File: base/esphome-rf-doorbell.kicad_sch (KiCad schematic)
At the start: 93 parts, among them J1 B4B-XH, J2 CONUFL001-SMD-T, J3 Conn_01x01, J4 Conn_01x01, SW1 Boot, U1 BQ25628E, U2 RFM69W, U3 TPS7A2033, U4 MAX17261xxTD, U5 TPS629206DRLR, U6 G3VM-31DR, U7 ESP32-S2-MINI-2, U8 G3VM-63ER, U9 TLP2391

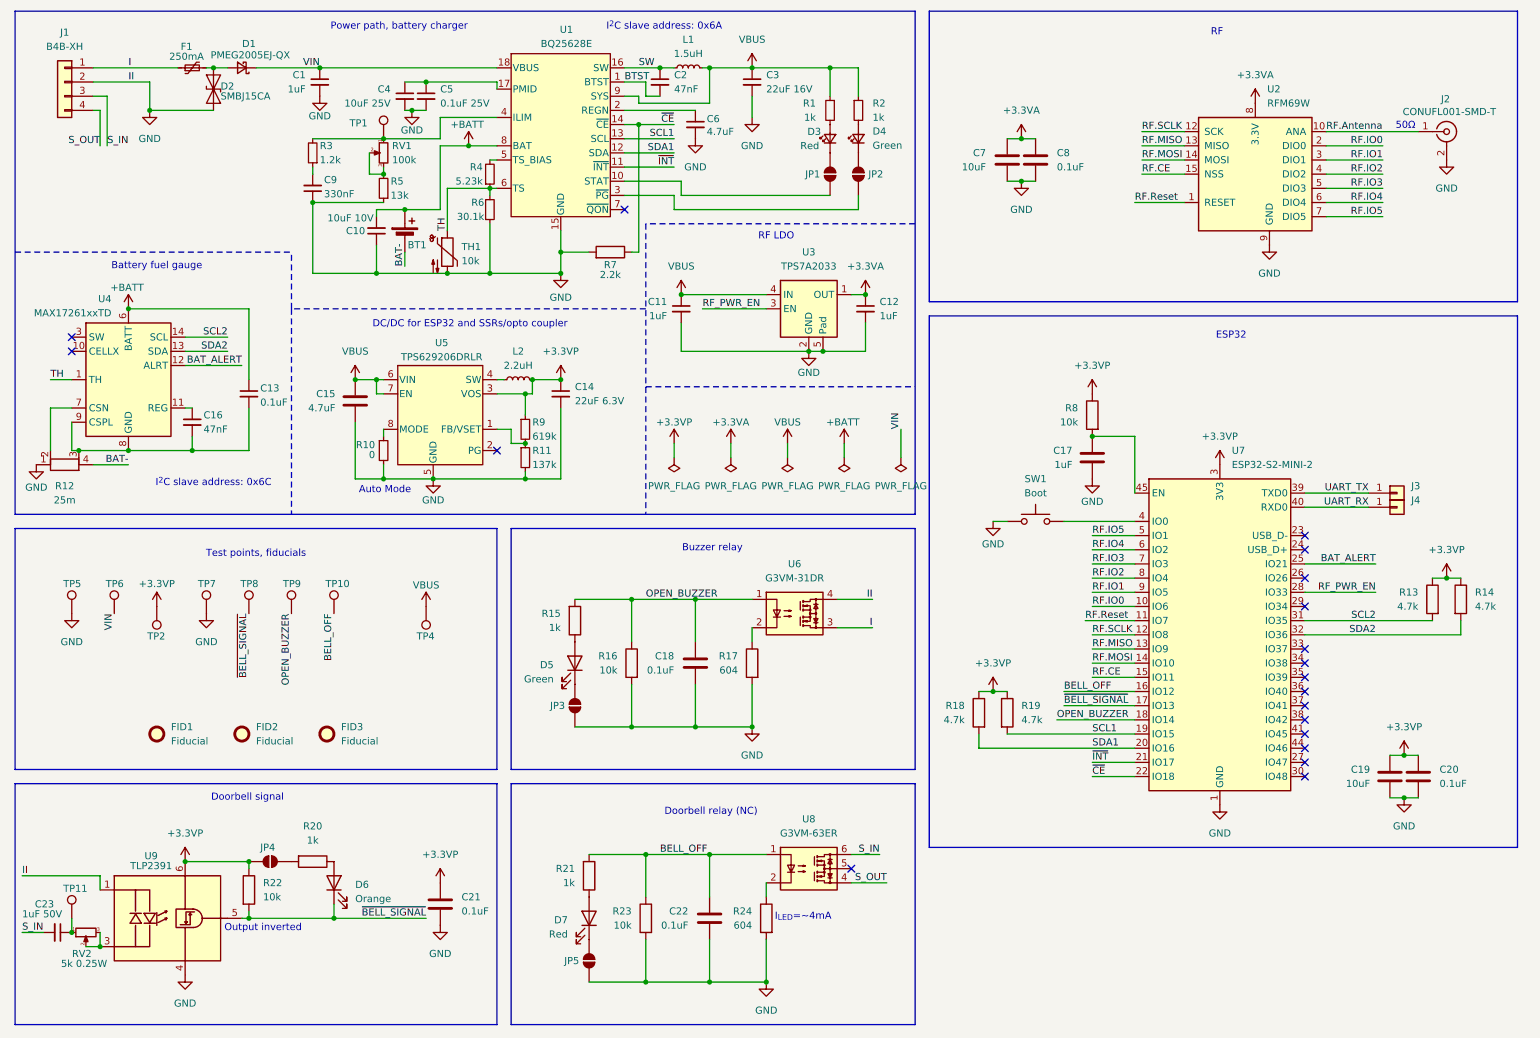
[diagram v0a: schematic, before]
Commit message: Base board Rev3
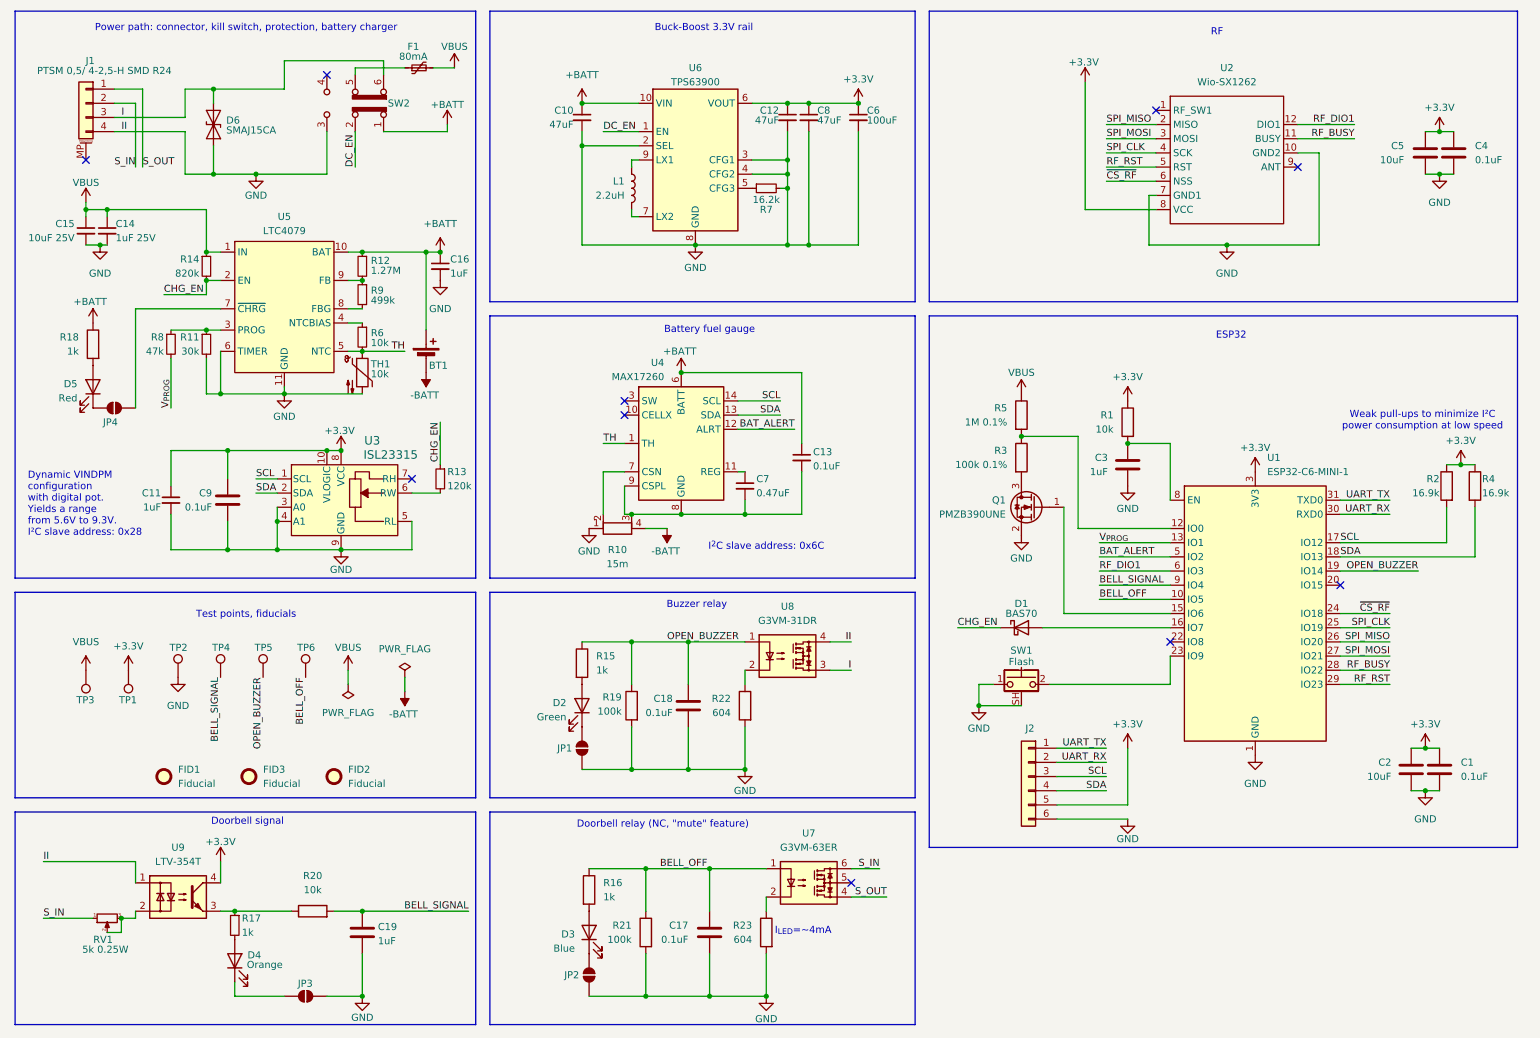
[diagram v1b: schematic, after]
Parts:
- removed C1: 1uF, Capacitor_SMD:C_0402_1005Metric, symbol Device:C_Small
- removed C15: 4.7uF, Capacitor_SMD:C_0603_1608Metric, symbol Device:C
- removed C2: 47nF, Capacitor_SMD:C_0402_1005Metric, symbol Device:C_Small
- removed C21: 0.1uF, Capacitor_SMD:C_0402_1005Metric, symbol Device:C
- removed C23: 1uF 50V, Capacitor_SMD:C_0805_2012Metric, symbol Device:C_Small
- removed C3: 22uF 16V, Capacitor_SMD:C_0805_2012Metric, symbol Device:C_Small
- removed C4: 10uF 25V, Capacitor_SMD:C_0603_1608Metric, symbol Device:C_Small
- removed C5: 0.1uF 25V, Capacitor_SMD:C_0402_1005Metric, symbol Device:C_Small
- removed C9: 330nF, Capacitor_SMD:C_0402_1005Metric, symbol Device:C_Small
- removed D1: PMEG2005EJ-QX, Diode_SMD:D_SOD-323F, symbol Device:D_Schottky_Small
- removed D3: Red, LED_SMD:LED_0603_1608Metric, symbol Device:LED_Small
- removed D4: Green, LED_SMD:LED_0603_1608Metric, symbol Device:LED_Small
- removed J1: B4B-XH, Connector_JST:JST_XH_B4B-XH-A_1x04_P2.50mm_Vertical, symbol Connector_Generic:Conn_01x04
- removed J2: CONUFL001-SMD-T, Connector_Coaxial:U.FL_Hirose_U.FL-R-SMT-1_Vertical, symbol Connector:Conn_Coaxial
- removed J3, J4: Conn_01x01, TestPoint:TestPoint_Keystone_5000-5004_Miniature, symbol Connector_Generic:Conn_01x01
- removed JP1, JP2: SolderJumper_2_Open, Jumper:SolderJumper-2_P1.3mm_Open_RoundedPad1.0x1.5mm, symbol Jumper:SolderJumper_2_Open
- removed L1: 1.5uH, Inductor_SMD:L_Wuerth_MAPI-4020, symbol Device:L_Small
- removed L2: 2.2uH, Inductor_SMD:L_1210_3225Metric, symbol Device:L_Small
- removed R1, R2: 1k, Resistor_SMD:R_0603_1608Metric, symbol Device:R_Small
- removed R10: 0, Resistor_SMD:R_0402_1005Metric, symbol Device:R_Small
- removed R13: 4.7k, Resistor_SMD:R_0402_1005Metric, symbol Device:R
- removed R14: 4.7k, Resistor_SMD:R_1206_3216Metric, symbol Device:R
- removed R20, R21: 1k, Resistor_SMD:R_0603_1608Metric, symbol Device:R
- removed R3: 1.2k, Resistor_SMD:R_0603_1608Metric, symbol Device:R_Small
- removed R4: 5.23k, Resistor_SMD:R_0402_1005Metric, symbol Device:R_Small
- removed R5: 13k, Resistor_SMD:R_0402_1005Metric, symbol Device:R_Small
- removed R7: 2.2k, Resistor_SMD:R_0603_1608Metric, symbol Device:R
- removed RV1: 100k, Potentiometer_SMD:Potentiometer_Bourns_TC33X_Vertical, symbol Device:R_Potentiometer_Small
- removed SW1: Boot, Button_Switch_SMD:SW_SPST_PTS647_Sx50, symbol Switch:SW_Push
- removed TP1, TP11, TP4, TP5: TestPoint, TestPoint:TestPoint_Pad_D1.5mm, symbol Connector:TestPoint
- removed U1: BQ25628E, lib:WQFN-HR18__RYK_TEX, symbol BQ25628E:BQ25628ERYKR
- removed U2: RFM69W, RF_Module:HOPERF_RFM69HW, symbol RF_Module:RFM69W
- removed U3: TPS7A2033, Package_SON:Texas_X2SON-4_1x1mm_P0.65mm, symbol Regulator_Linear:TPS7A20xxxDQN
- removed U5: TPS629206DRLR, lib:SOT5X3-8_DRL_TEX, symbol TPS629206:TPS629206DRLR
- removed U7: ESP32-S2-MINI-2, RF_Module:ESP32-S2-MINI-1, symbol RF_Module:ESP32-S3-MINI-1
- removed U9: TLP2391, lib:OPTO_TLP2367_TPR_E, symbol Isolator:TLP2310
- added C15: 10uF 25V, Capacitor_SMD:C_0603_1608Metric, symbol Device:C_Small
- added C16: 1uF, Capacitor_SMD:C_0402_1005Metric, symbol Device:C_Small
- added C19: 1uF, Capacitor_SMD:C_0402_1005Metric, symbol Device:C
- added C8: 47uF, Capacitor_SMD:C_0805_2012Metric, symbol Device:C_Small
- added C9: 0.1uF, Capacitor_SMD:C_0402_1005Metric, symbol Device:C
- added D1: BAS70, Diode_SMD:D_SOD-523, symbol Device:D_Schottky
- added D5: Red, LED_SMD:LED_0603_1608Metric, symbol Device:LED
- added J1: PTSM 0,5/ 4-2,5-H SMD R24, lib:PHOENIX_1702474, symbol Connector_Generic_MountingPin:Conn_01x04_MountingPin
- added J2: Conn_01x06, lib:Connector_PogoClamp_1.27mm, symbol Connector_Generic:Conn_01x06
- added JP4: SolderJumper_2_Open, Jumper:SolderJumper-2_P1.3mm_Open_RoundedPad1.0x1.5mm, symbol Jumper:SolderJumper_2_Open
- added L1: 2.2uH, Inductor_SMD:L_1210_3225Metric, symbol Device:L
- added Q1: PMZB390UNE, Package_DFN_QFN:Diodes_DFN1006-3, symbol Transistor_FET:2N7002
- added R12: 1.27M, Resistor_SMD:R_0402_1005Metric, symbol Device:R_Small
- added R13: 120k, Resistor_SMD:R_0402_1005Metric, symbol Device:R_Small
- added R14: 820k, Resistor_SMD:R_0805_2012Metric, symbol Device:R_Small
- added R16, R18: 1k, Resistor_SMD:R_0402_1005Metric, symbol Device:R
- added R17: 1k, Resistor_SMD:R_0402_1005Metric, symbol Device:R_Small
- added R3: 100k 0.1%, Capacitor_SMD:C_0402_1005Metric, symbol Device:R
- added R5: 1M 0.1%, Capacitor_SMD:C_0402_1005Metric, symbol Device:R
- added R7: 16.2k, Resistor_SMD:R_0402_1005Metric, symbol Device:R_Small
- added R8: 47k, Resistor_SMD:R_0402_1005Metric, symbol Device:R_Small
- added SW1: Flash, Button_Switch_SMD:SW_SPST_Panasonic_EVQPL_3PL_5PL_PT_A08, symbol Switch:SW_Push_Shielded
- added SW2: CL-SB-22A-11T, lib:CL-SB-22A, symbol Switch:SW_Slide_DPDT
- added U1: ESP32-C6-MINI-1, lib:XCVR_ESP32-C6-MINI-1U-N4, symbol RF_Module:ESP32-C6-MINI-1
- added U2: Wio-SX1262, lib:Wio-SX1262 PCB Package, symbol Wio-SX1262 Schematic Package:MODULE-WIO-SX1262
- added U3: ISL23315, lib:L10_2P1X1P6A_INR, symbol ISL23315:ISL23315TFRUZ-T7A
- added U5: LTC4079, Package_DFN_QFN:DFN-10-1EP_3x3mm_P0.5mm_EP1.65x2.38mm, symbol LTC4079:LTC4079
- added U6: TPS63900, Package_SON:WSON-10-1EP_2.5x2.5mm_P0.5mm_EP1.2x2mm_ThermalVias, symbol Regulator_Switching:TPS63900
- added U9: LTV-354T, Package_SO:SO-4_4.4x3.6mm_P2.54mm, symbol Isolator:LTV-354T
- BT1: MPN ICP422339PR -> 532610271
- C10: value 10uF 10V -> 47uF; footprint Capacitor_SMD:C_0603_1608Metric -> Capacitor_SMD:C_0805_2012Metric
- C12: value 1uF -> 47uF; footprint Capacitor_SMD:C_0402_1005Metric -> Capacitor_SMD:C_0805_2012Metric
- C14: value 22uF 6.3V -> 1uF 25V; footprint Capacitor_SMD:C_0603_1608Metric -> Capacitor_SMD:C_0402_1005Metric
- C6: value 4.7uF -> 100uF; footprint Capacitor_SMD:C_0603_1608Metric -> Capacitor_SMD:C_1206_3216Metric
- C7: renamed from C16; value 47nF -> 0.47uF
- D3: renamed from D7; value Red -> Blue
- D6: renamed from D2; value SMBJ15CA -> SMAJ15CA; footprint Diode_SMD:D_SMB -> Diode_SMD:D_SMA; MPN SMBJ15CA -> SMAJ15CA
- F1: value 250mA -> 80mA; footprint Fuse:Fuse_1206_3216Metric -> Fuse:Fuse_0603_1608Metric; MPN SMD1206B025TF/24 -> SMD0603B008TF
- R10: renamed from R12; value 25m -> 15m; footprint Resistor_SMD:R_Shunt_Vishay_WSK2512_6332Metric_T1.19mm -> lib:R_Shunt_D1WRL1206; MPN WSK2512R0250DEA -> D1WRL1206L4R015D-T5
- R11: value 137k -> 30k; footprint Resistor_SMD:R_0603_1608Metric -> Resistor_SMD:R_0402_1005Metric
- R15: footprint Resistor_SMD:R_0603_1608Metric -> Resistor_SMD:R_0402_1005Metric
- R19: renamed from R16; value 10k -> 100k; footprint Resistor_SMD:R_0603_1608Metric -> Resistor_SMD:R_0402_1005Metric
- R2: renamed from R18; value 4.7k -> 16.9k; footprint Resistor_SMD:R_1206_3216Metric -> Resistor_SMD:R_0402_1005Metric
- R20: renamed from R22; footprint Resistor_SMD:R_0603_1608Metric -> Resistor_SMD:R_0402_1005Metric
- R21: renamed from R23; value 10k -> 100k; footprint Resistor_SMD:R_0603_1608Metric -> Resistor_SMD:R_0402_1005Metric
- R4: renamed from R19; value 4.7k -> 16.9k
- R6: value 30.1k -> 10k
- R9: value 619k -> 499k; footprint Resistor_SMD:R_0603_1608Metric -> Resistor_SMD:R_0402_1005Metric
- TH1: footprint Resistor_THT:R_Axial_DIN0204_L3.6mm_D1.6mm_P5.08mm_Vertical -> Resistor_SMD:R_0603_1608Metric; MPN MF52A103J3435 (A1) -> NTCS0603E3103FLT
- TP1: renamed from TP2; footprint TestPoint:TestPoint_Keystone_5000-5004_Miniature -> TestPoint:TestPoint_Pad_D1.5mm
- TP2: renamed from TP7; footprint TestPoint:TestPoint_Keystone_5000-5004_Miniature -> TestPoint:TestPoint_Pad_D1.5mm
- U4: value MAX17261xxTD -> MAX17260
- renumbered C20 to C1, C22 to C17, C19 to C2, C17 to C3, C8 to C4, C7 to C5, D5 to D2, D6 to D4, FID3 to FID2, FID2 to FID3, JP3 to JP1, JP5 to JP2, JP4 to JP3, R8 to R1, R17 to R22, R24 to R23, RV2 to RV1, TP6 to TP3, TP8 to TP4, TP9 to TP5, TP10 to TP6, U8 to U7, U6 to U8
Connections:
- net +3.3VA is gone; now on net +3.3V: C12.1, C4.1, C5.1
- net SDA1 is gone; now on net SCL: R2.2
- net SDA2 is gone; now on net SDA: U4.13 (SDA)
- net VIN is gone; now on net VBUS: TP3.1
- net +BATT: now also C10.1, C16.1, R12.1, R18.1, SW2.1 (A), U5.10 (BAT), U6.10 (VIN); no longer C10.2
- net BAT_ALERT: now also U1.5 (IO2)
- net BELL_OFF: now also R16.1, U1.10 (IO5)
- net GND: now also C10.2, JP3.2 (B), C15.2, C16.2, C19.2, C8.2, C9.2, J1.4 (Pin_4), J2.6 (Pin_6), Q1.2 (S), R7.2, SW1.1, SW1.SH (B), SW2.3 (C), U1.1 (GND), U1.11 (GND), U1.14 (GND), U1.2 (GND), U1.36 (GND), U1.37 (GND), U1.38 (GND), U1.39 (GND), U1.40 (GND), U1.41 (GND), U1.42 (GND), U1.43 (GND), U1.44 (GND), U1.45 (GND), U1.46 (GND), U1.47 (GND), U1.48 (GND), U1.49 (GND), U1.50 (GND), U1.51 (GND), U1.52 (GND), U1.53 (GND), U2.10 (GND2), U2.7 (GND1), U3.3 (A0), U3.4 (A1), U3.5 (RL), U3.9 (GND), U5.11 (GND), U5.6 (TIMER), U6.11 (GND), U6.2 (SEL), U6.3 (CFG1), U6.4 (CFG2), U6.8 (GND), U9.1; no longer C10.1, R6.1
- net I: now also D6.2 (A2), J1.3 (Pin_3), SW2.6 (C); no longer F1.1
- net OPEN_BUZZER: now also R15.1, U1.19 (IO14); no longer R15.2
- net S_IN: now also RV1.1, J1.2 (Pin_2)
- net S_OUT: now also J1.1 (Pin_1)
- net TH: now also U5.5 (NTC)
- net UART_RX: now also J2.2 (Pin_2), U1.30 (RXD0)
- net UART_TX: now also J2.1 (Pin_1), U1.31 (TXD0)
- net VBUS: now also C14.1, F1.2, C15.1, R14.1, R5.1, U5.1 (IN); no longer C11.1
- net +3.3V: now reaches C6.1
- net +3.3V: now also C1.1, C11.1, C2.1, R1.1, R2.1, R4.1, TP1.1, C8.1, C9.1, J2.5 (Pin_5), U1.3 (3V3), U2.8 (VCC), U3.10 (VLOGIC), U3.8 (VCC), U6.6 (VOUT), U9.4
- net at RV1.2, RV1.3: now also U9.2
- net at D4.2 (A): now also R17.2
- net at JP3.1 (A): now also D4.1 (K)
- net at C3.1, R1.2: now also U1.8 (EN)
- net at D3.2 (A): now also R16.2
- net at R9.2: now also U5.8 (FBG); no longer R11.1
- net at D2.2 (A): now also R15.2; no longer R15.1
- removed net +3.3VP: C1.1, C14.1, C2.1, JP3.2 (B), R1.1, R2.1, R20.1, R4.1, R9.1, TP1.1
- net BAT- renamed -BATT
- net SCL1 renamed SDA
- net SDA: now also J2.4 (Pin_4), U1.18 (IO13), U3.2 (SDA)
- net SCL2 renamed SCL
- net SCL: now also J2.3 (Pin_3), U1.17 (IO12), U3.1 (SCL)
- net ~{BELL_SIGNAL} renamed BELL_SIGNAL
- net BELL_SIGNAL: now also C19.1, U1.9 (IO4); no longer D4.1 (K)
- new net: R12.2, R9.1, U5.9 (FB)
- new net: F1.1, SW2.5 (B)
- new net: R13.2, U3.6 (RW)
- new net: L1.1, U6.9 (LX1)
- new net: L1.2, U6.7 (LX2)
- new net: R3.1, R5.2, U1.12 (IO0)
- new net: Q1.1 (G), U1.15 (IO6)
- new net: D1.2 (A), U1.16 (IO7)
- new net: SW1.2, U1.23 (IO9)
- new net: D5.1 (K), JP4.2 (B)
- new net: D5.2 (A), R18.2
- new net: R11.1, R8.1, U5.3 (PROG)
- new net: R7.1, U6.5 (CFG3)
- new net: Q1.3 (D), R3.2
- new net: R17.1, R20.1, U9.3
- new net: R6.1, U5.4 (NTCBIAS)
- new net: JP4.1 (A), U5.7 (~{CHRG})
- new net CHG_EN: D1.1 (K), R13.1, R14.2, U5.2 (EN)
- new net DC_EN: SW2.2 (B), U6.1 (EN)
- new net RF_BUSY: U1.28 (IO22), U2.11 (BUSY)
- new net RF_DIO1: U1.6 (IO3), U2.12 (DIO1)
- new net RF_RST: U1.29 (IO23), U2.5 (RST)
- new net SPI_CLK: U1.25 (IO19), U2.4 (SCK)
- new net SPI_MISO: U1.26 (IO20), U2.2 (MISO)
- new net SPI_MOSI: U1.27 (IO21), U2.3 (MOSI)
- new net V_{PROG}: R8.2, U1.13 (IO1)
- new net ~{CS_RF}: U1.24 (IO18), U2.6 (NSS)
- no-connect marks 19 -> 10
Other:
- note added: "Buck-Boost 3.3V rail"
- note added: "Doorbell relay (NC, "mute" feature)"
- note added: "Dynamic VINDPM configuration with digital pot. Yields a range from 5.6V to 9.3V. I²C slave address: 0x28"
- note added: "Power path: connector, kill switch, protection, battery charger"
- note added: "Weak pull-ups to minimize I²C power consumption at low speed"
- note removed: "50Ω"
- note removed: "Auto Mode"
- note removed: "DC/DC for ESP32 and SSRs/opto coupler"
- note removed: "Doorbell relay (NC)"
- note removed: "I^{2}C slave address: 0x6A"
- note removed: "Output inverted"
- note removed: "Power path, battery charger"
- note removed: "RF LDO"
- moved on the sheet: BT1, C1, C13, C17, C18, C2, C3, C4, C5, C7, D2, D3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
